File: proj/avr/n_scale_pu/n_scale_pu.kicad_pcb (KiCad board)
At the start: 2 copper layers, 48 x 28 mm, 38 parts, among them J1 USB_C_Receptacle_USB2.0_16P, J2 UPDI, J3 feeder, SW1 SW_Push, SW2 SW_Push, SW3 SW_Push, SW4 SW_Push, U1 CH221K, U2 AP7375, U3 ATtiny1604-SS, U4 AQM0802A-RN-GBW, U5 AM2837

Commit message: -
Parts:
- R5: value 4k7 -> 10k
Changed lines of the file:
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@@
 		)
 		(fp_rect
+			(start -15.8 -3)
+			(end -15 3)
+			(stroke
+				(width 0.1)
+				(type solid)
+			)
+			(fill no)
+			(layer "F.Fab")
+		)
+		(fp_rect
 			(start -15 -6.75)
 			(end 15 12.75)
@@
 			)
 		)
+		(fp_text user "BACKLIGHT_LENS"
+			(at -15.4 0 270)
+			(unlocked yes)
+			(layer "F.Fab")
+			(effects
+				(font
+					(size 0.4 0.4)
+					(thickness 0.05)
+				)
+			)
+		)
 		(pad "1" thru_hole roundrect
 			(at -6 12.9)
@@
 			)
 		)
-		(property "Value" "4k7"
+		(property "Value" "10k"
 			(at 0 -1.43 90)
 			(layer "B.Fab")
@@
 		)
 	)
-	(gr_text "4k7"
+	(gr_text "10k"
 		(at 101.8 93.4 0)
 		(layer "B.Mask")

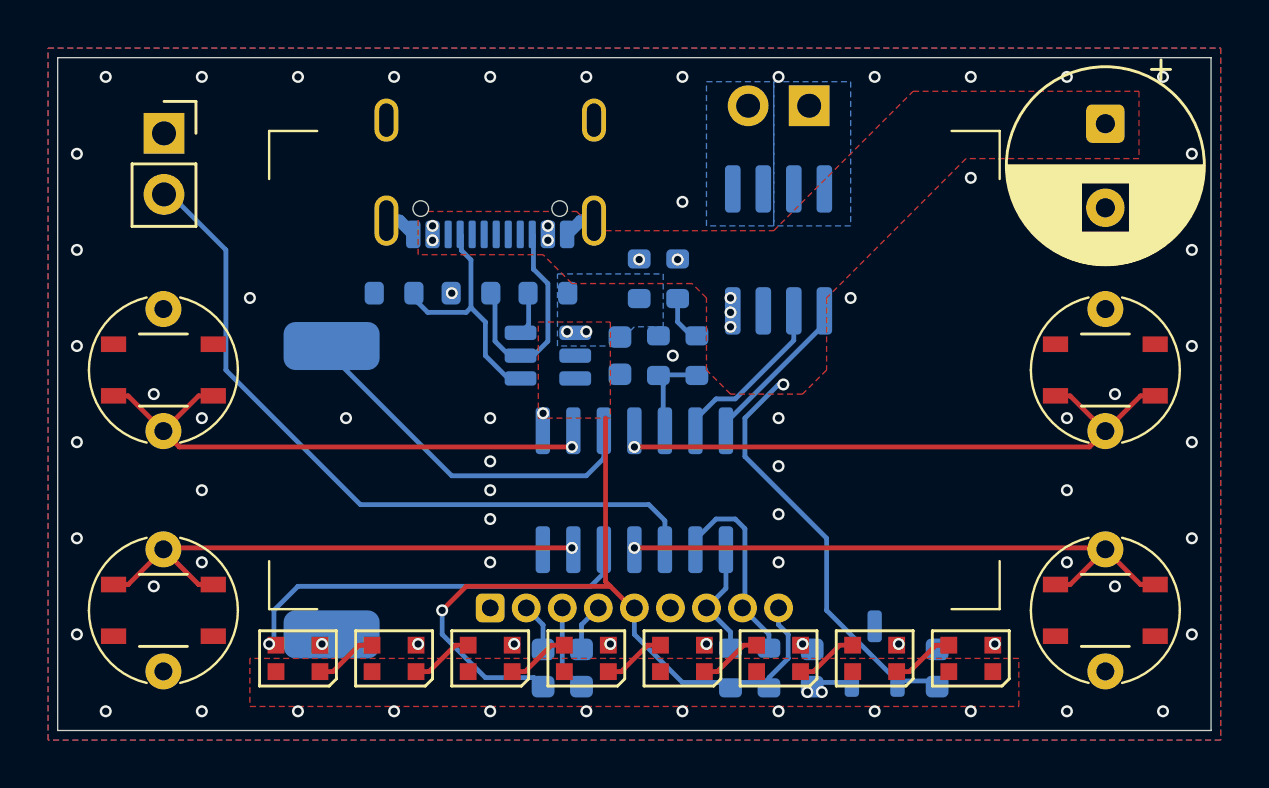
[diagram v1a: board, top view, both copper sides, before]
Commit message: -
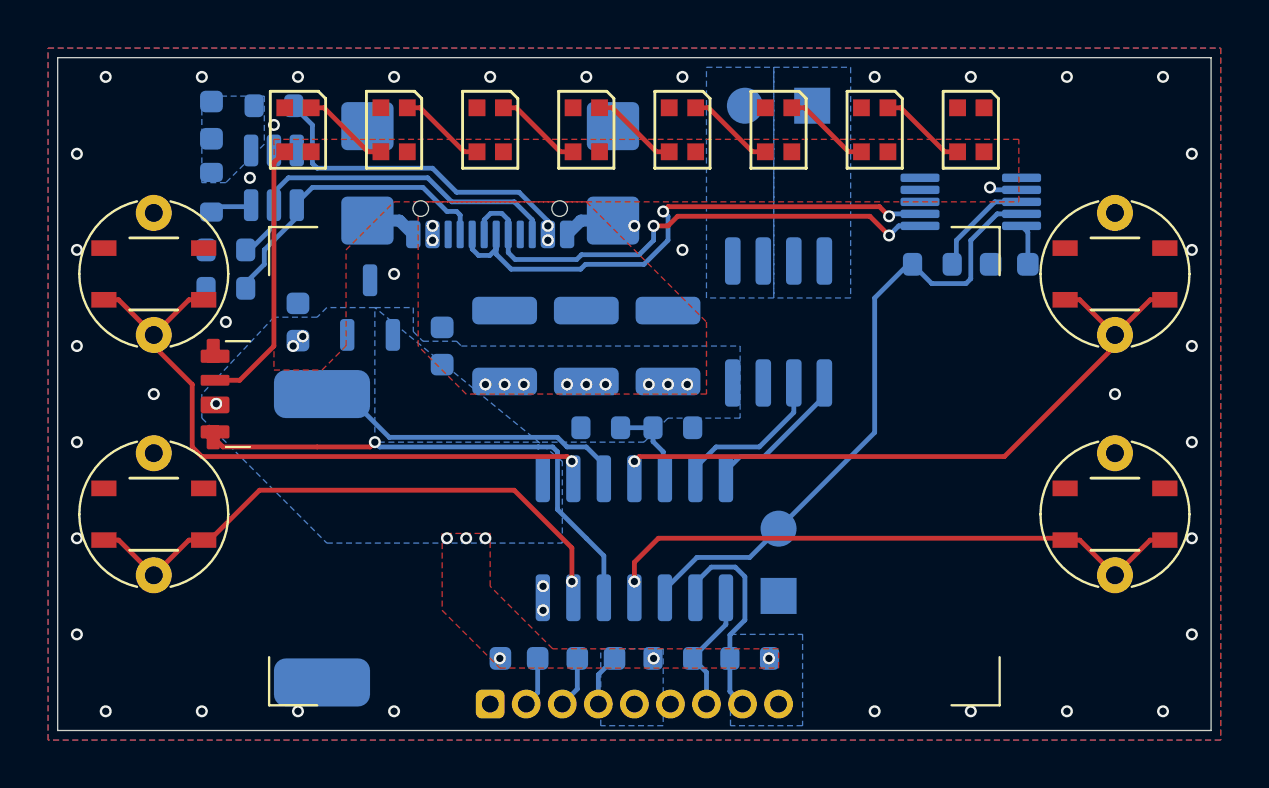
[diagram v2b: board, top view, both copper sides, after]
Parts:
- removed the C1 at (119.6, 88.7)
- removed J2: UPDI, Connector_PinSocket_2.54mm:PinSocket_1x02_P2.54mm_Vertical
- removed J3: feeder, Connector_PinHeader_2.54mm:PinHeader_1x02_P2.54mm_Vertical
- removed the R6 at (102.6, 98.4)
- added C2: 0u1, Capacitor_SMD:C_0603_1608Metric, B.Cu at (115.6, 94.6)
- added C5: 47u, Capacitor_SMD:C_1210_3225Metric, B.Cu at (101.4, 98.0)
- added C6: 47u, Capacitor_SMD:C_1210_3225Metric, B.Cu at (98.0, 98.0)
- added C7: 47u, Capacitor_SMD:C_1210_3225Metric, B.Cu at (94.6, 98.0)
- added D1: SK6112-SIDE-RG-A, Library:SK6112-SIDE-RG-A, F.Cu at (84.0, 100.0)
- added R4: 4k7, Resistor_SMD:R_0603_1608Metric, B.Cu at (112.4, 94.6)
- added TP1: GND, TestPoint:TestPoint_Pad_1.5x1.5mm, B.Cu at (106.0, 108.4)
- added TP2: UPDI, TestPoint:TestPoint_Pad_D1.5mm, B.Cu at (106.0, 105.6)
- added TP3: OUT_A, TestPoint:TestPoint_Pad_1.5x1.5mm, B.Cu at (107.4, 88.0)
- added TP4: OUT_B, TestPoint:TestPoint_Pad_D1.5mm, B.Cu at (104.6, 88.0)
- added U1: CH340E, Package_SO:MSOP-10_3x3mm_P0.5mm, B.Cu at (114.0, 92.0)
- J1: footprint Connector_USB:USB_C_Receptacle_GCT_USB4105-xx-A_16P_TopMnt_Horizontal -> Connector_USB:USB_C_Receptacle_GCT_USB4110
- moved C4 25.8 mm to (86.0, 97.0)
- moved U2 25.5 mm to (89.0, 96.4)
- moved C1 24.6 mm to (92.0, 98.0)
- moved D2 22.0 mm to (86.0, 89.0), turned to -90 degrees
- moved D3 22.0 mm to (90.0, 89.0), turned to -90 degrees
- moved D4 22.0 mm to (94.0, 89.0), turned to -90 degrees
- moved D5 22.0 mm to (98.0, 89.0), turned to -90 degrees
- moved D6 22.0 mm to (102.0, 89.0), turned to -90 degrees
- moved D7 22.0 mm to (106.0, 89.0), turned to -90 degrees
- moved D8 22.0 mm to (110.0, 89.0), turned to -90 degrees
- moved D9 22.0 mm to (114.0, 89.0), turned to -90 degrees
- moved C3 19.6 mm to (82.4, 88.6), turned to 90 degrees
- moved R3 16.8 mm to (85.0, 88.0), turned to 180 degrees
- moved R5 14.6 mm to (82.4, 91.6), turned to -90 degrees
- moved U3 13.6 mm to (85.0, 91.0), turned to -90 degrees
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- renumbered C3 to C1, C2 to C3, C5 to C8, C6 to C9, D1 to D2, D2 to D3, D3 to D4, D4 to D5, D5 to D6, D6 to D7, D7 to D8, D8 to D9, R4 to R5, R5 to R6, U1 to U3, U3 to U4, U4 to U5, U5 to U6
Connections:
- net SCL_3V3 renamed SCL
- net SDA_3V3 renamed SDA
- C8 pad 1: +3V3 -> +5V
- D2 pad 3: NP -> Net-(D1-DOUT)
- J1 pad A6: unconnected-(J1-D+-PadA6) -> D+
- J1 pad A7: unconnected-(J1-D--PadA7) -> D-
- J1 pad B6: unconnected-(J1-D+-PadB6) -> D+
- J1 pad B7: unconnected-(J1-D--PadB7) -> D-
- R6 pad 2: Net-(R5-Pad2) -> V_SENSE
- R8 pad 1: +3V3 -> +5V
- R9 pad 1: +3V3 -> +5V
- U4 pad 1: +3V3 -> +5V
- U5 pad 5: +3V3 -> +5V
- U5 pad 9: +3V3 -> +5V
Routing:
- net +3V3: track 33.6 -> 0.00 mm, vias 4 -> 0
- net D-: track 0.00 -> 23.4 mm, vias 0 -> 2
- net D+: track 0.00 -> 22.0 mm, vias 0 -> 2
- net Net-(D1-DOUT): track 0.00 -> 11.3 mm
- net CC2: track 9.48 -> 15.3 mm
- net NP: track 16.8 -> 21.6 mm
- net Net-(U1-TXD): track 0.00 -> 4.45 mm
- net BTN1: track 22.6 -> 26.7 mm
- net UPDI: track 30.6 -> 26.5 mm
- net VBUS: track 17.5 -> 14.1 mm, vias 10 -> 13
- net BTN3: track 25.2 -> 27.8 mm
- net CC1: track 10.3 -> 12.8 mm
- net Net-(R5-Pad2): track 2.01 -> 0.00 mm
- net SPK: track 15.2 -> 13.5 mm
- net Net-(U1-V3): track 0.00 -> 1.71 mm
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- added copper zone on B.Cu, net +5V
- added copper zone on B.Cu, net VBUS
- removed copper zone on F.Cu, net +3V3
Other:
- board text added: "0u1"
- board text added: "47u *3"
- board text added: "CH340E"
- board text added: "PKLCS1212E 4001-R1"
- board text added: "SK6112-SIDE-RG-A"
- board text added: "USB4110"
- board text added: "↑ WS2812C-2020 *8 ↑"
- board text added: "↓ AQM0802A-RN-GBW ↓"
- board text removed: "470u"
- board text removed: "AQM0802A-RN-GBW"
- board text removed: "PA3"
- board text removed: "PKLCS1212E4001-R1"
- board text removed: "USB4105"
- board text removed: "WS2812C-2020"
